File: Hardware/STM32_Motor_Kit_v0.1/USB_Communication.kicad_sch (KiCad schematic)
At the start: 7 parts, among them J8 USB_B_Mini, U17 TVS_Diode_USB

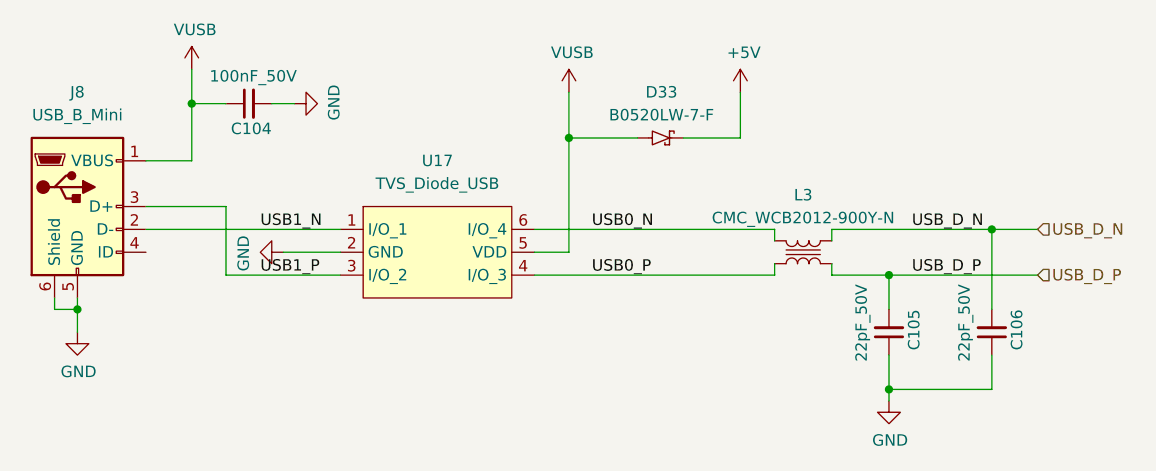
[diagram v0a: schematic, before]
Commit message: 12.01.2025
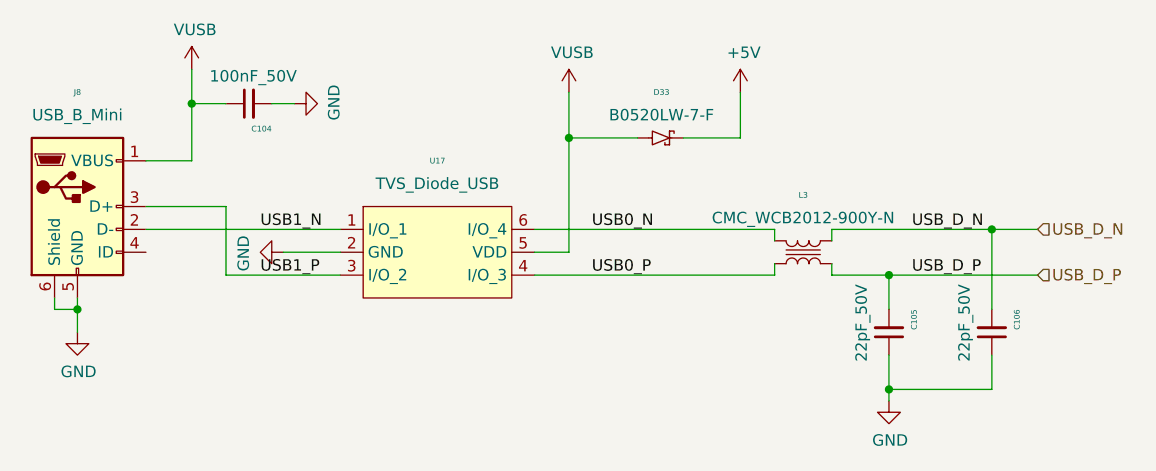
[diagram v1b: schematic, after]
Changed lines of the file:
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@@
 			(effects
 				(font
-					(size 1.27 1.27)
+					(face "Arial")
+					(size 0.635 0.635)
 				)
 			)
@@
 			(effects
 				(font
-					(size 1.27 1.27)
+					(face "Arial")
+					(size 0.635 0.635)
 				)
 				(hide yes)
@@
 			(effects
 				(font
-					(size 1.27 1.27)
+					(face "Arial")
+					(size 0.635 0.635)
 				)
 			)
@@
 			(effects
 				(font
-					(size 1.27 1.27)
+					(face "Arial")
+					(size 0.635 0.635)
 				)
 				(hide yes)
@@
 			(effects
 				(font
-					(size 1.27 1.27)
+					(face "Arial")
+					(size 0.635 0.635)
 				)
 				(hide yes)
@@
 			(effects
 				(font
-					(size 1.27 1.27)
+					(face "Arial")
+					(size 0.635 0.635)
 				)
 			)
@@
 			(effects
 				(font
-					(size 1.27 1.27)
+					(face "Arial")
+					(size 0.635 0.635)
 				)
 				(hide yes)
@@
 			(effects
 				(font
-					(size 1.27 1.27)
+					(face "Arial")
+					(size 0.635 0.635)
 				)
 				(hide yes)
@@
 			(effects
 				(font
-					(size 1.27 1.27)
+					(face "Arial")
+					(size 0.635 0.635)
 				)
 				(justify left)
@@
 			(effects
 				(font
-					(size 1.27 1.27)
+					(face "Arial")
+					(size 0.635 0.635)
 				)
 			)
@@
 			(effects
 				(font
-					(size 1.27 1.27)
+					(face "Arial")
+					(size 0.635 0.635)
 				)
 				(justify left)
@@
 			(effects
 				(font
-					(size 1.27 1.27)
+					(face "Arial")
+					(size 0.635 0.635)
 				)
 				(justify left)
@@
 			(effects
 				(font
-					(size 1.27 1.27)
+					(face "Arial")
+					(size 0.635 0.635)
 				)
 				(hide yes)
@@
 			(effects
 				(font
-					(size 1.27 1.27)
-				)
-				(hide yes)
+					(face "Arial")
+					(size 0.635 0.635)
+				)
+				(hide yes)

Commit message: Şema üzerinde değişiklikler devam ediyor
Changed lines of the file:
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@@
 (kicad_sch
-	(version 20231120)
+	(version 20250114)
 	(generator "eeschema")
-	(generator_version "8.0")
+	(generator_version "9.0")
 	(paper "A4")
 	(junction
@@
 	(label "USB1_N"
 		(at 76.2 82.55 0)
-		(fields_autoplaced yes)
 		(effects
 			(font
@@
 	(label "USB0_P"
 		(at 113.03 87.63 0)
-		(fields_autoplaced yes)
 		(effects
 			(font
@@
 	(label "USB0_N"
 		(at 113.03 82.55 0)
-		(fields_autoplaced yes)
 		(effects
 			(font
@@
 	(label "USB_D_N"
 		(at 148.59 82.55 0)
-		(fields_autoplaced yes)
 		(effects
 			(font
@@
 	(label "USB1_P"
 		(at 76.2 87.63 0)
-		(fields_autoplaced yes)
 		(effects
 			(font
@@
 	(label "USB_D_P"
 		(at 148.59 87.63 0)
-		(fields_autoplaced yes)
 		(effects
 			(font
@@
 		(shape input)
 		(at 162.56 87.63 0)
-		(fields_autoplaced yes)
 		(effects
 			(font
@@
 		(shape input)
 		(at 162.56 82.55 0)
-		(fields_autoplaced yes)
-		(effects
-			(font
+		(effects
+			(font
